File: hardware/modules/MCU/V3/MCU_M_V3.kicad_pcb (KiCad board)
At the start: 4 copper layers, 26.9 x 19 mm, 36 parts, among them J1 M50-3530242, J2 M50-3530342, Q1 IRLML6246TRPBF, U1 STM32F405OGYx, U2 STULPI01B, Y11 NX3225GA-10.000M-STD-CRG-2, Y12 FX135A-327

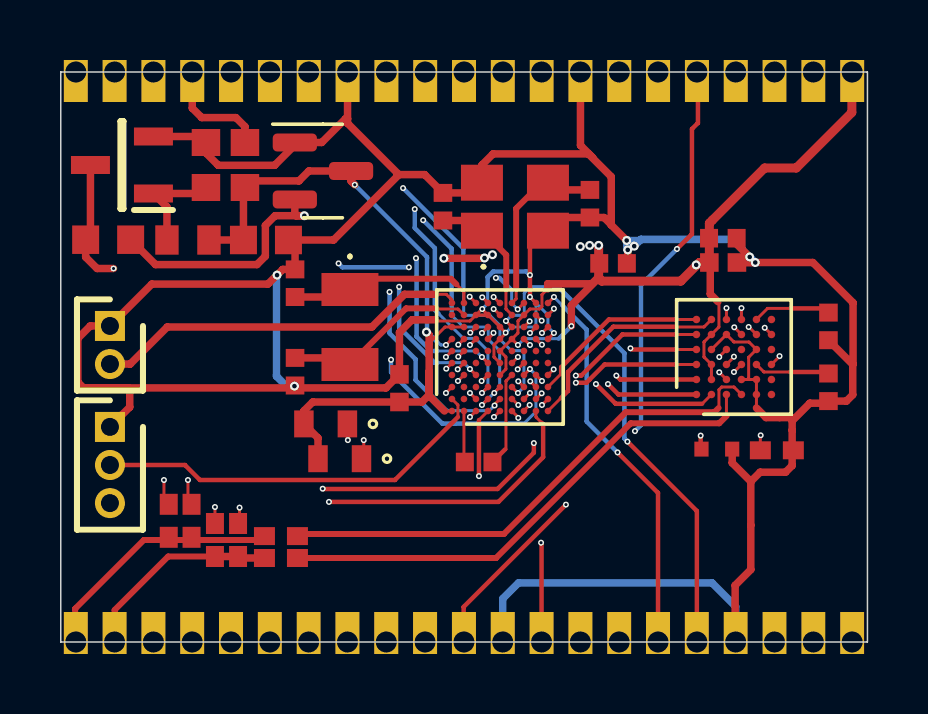
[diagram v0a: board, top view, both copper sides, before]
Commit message: MCU_V3 fix1
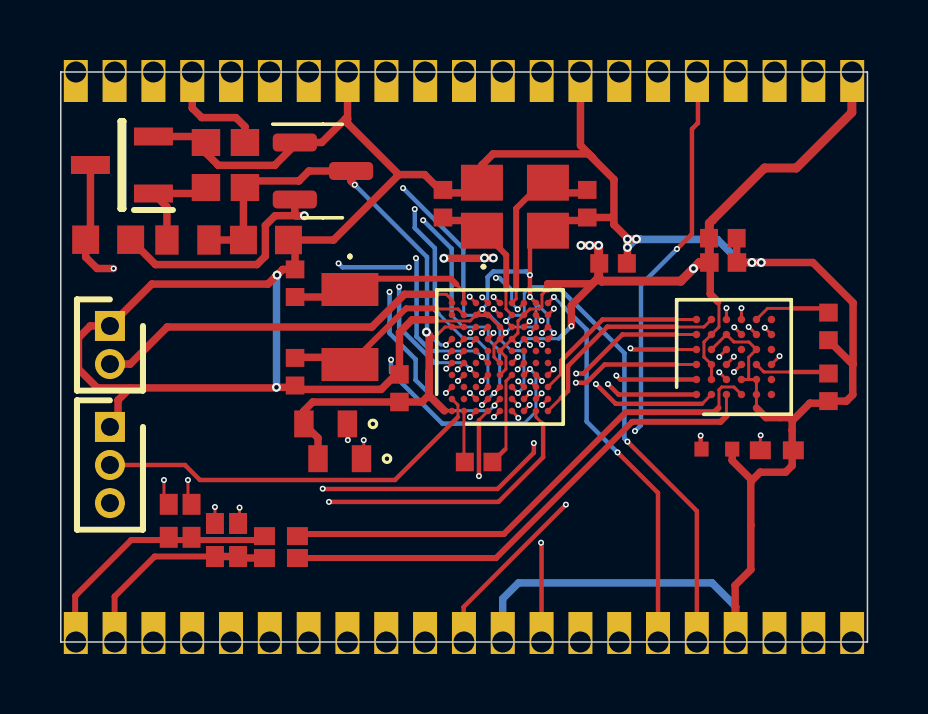
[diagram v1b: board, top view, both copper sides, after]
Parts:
- moved C12 0.10 mm to (183.2, 90.0)
- moved C13 0.09 mm to (188.0, 90.0)
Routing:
- net GND: track 124.9 -> 122.1 mm
- net /+3.3: track 68.1 -> 68.9 mm

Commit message: MCU_V3 fix2
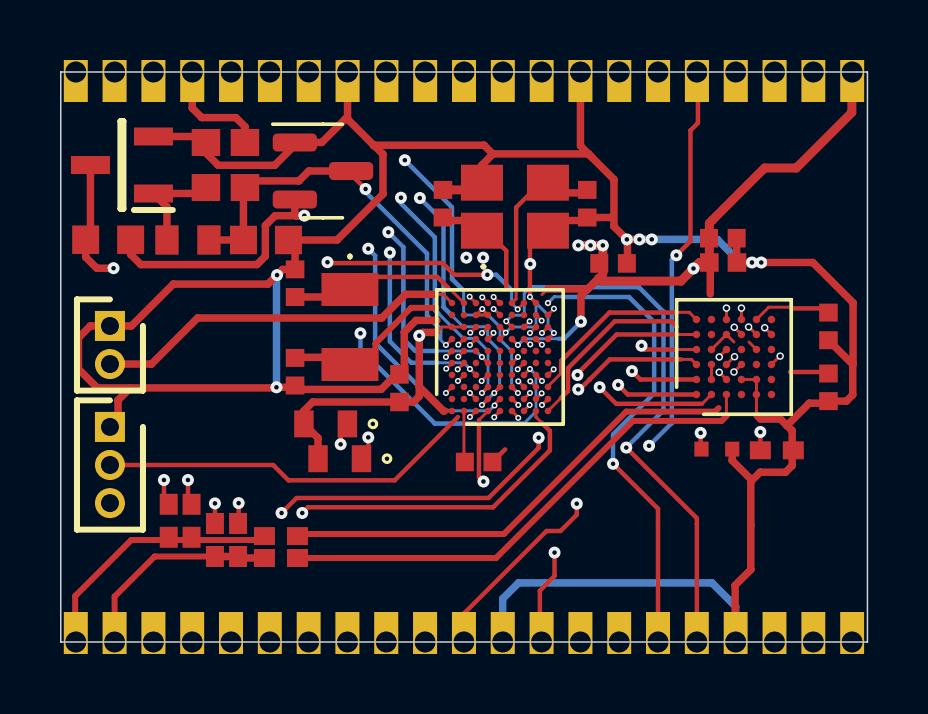
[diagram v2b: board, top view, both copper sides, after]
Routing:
- net /+3.3: track 68.9 -> 62.3 mm, vias 12 -> 9
- net GND: track 122.1 -> 116.5 mm
- net /M2_D1: track 16.6 -> 19.2 mm
- net /M2_D2: track 13.2 -> 15.8 mm
- net Net-(C11-Pad1): track 3.19 -> 0.62 mm
- net /M2_D8: track 18.8 -> 20.8 mm
- net /ULPI_XI: track 11.2 -> 9.64 mm
- net Net-(R25-Pad2): track 17.3 -> 15.8 mm
- net Net-(U2-PadE3): track 2.52 -> 1.23 mm
- net /ULPI_D6: track 7.30 -> 6.06 mm
- net Net-(C12-Pad2): track 4.67 -> 3.83 mm
- net Net-(C15-Pad1): track 6.74 -> 6.01 mm
- net /B4: track 14.4 -> 15.1 mm
- net /M1_D5: track 19.1 -> 18.4 mm
- net /SW_CLK: track 13.4 -> 12.7 mm
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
